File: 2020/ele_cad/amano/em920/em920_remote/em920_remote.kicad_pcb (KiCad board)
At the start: 2 copper layers, 40.6 x 58.4 mm, 8 parts, among them SW1 SW_Push, U1 ATtiny85-20PU, U2 TY92SS

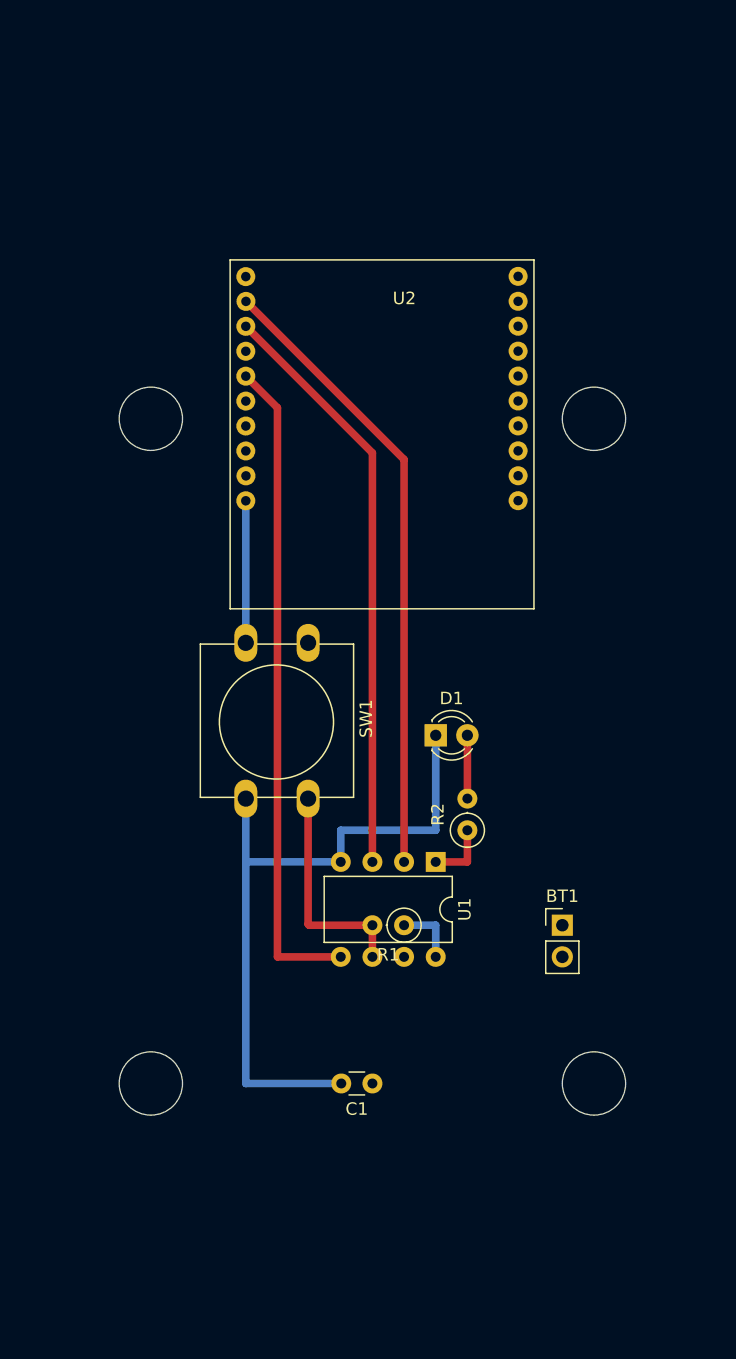
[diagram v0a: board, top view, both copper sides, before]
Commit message: 緊急停止リモコンのデータ更新
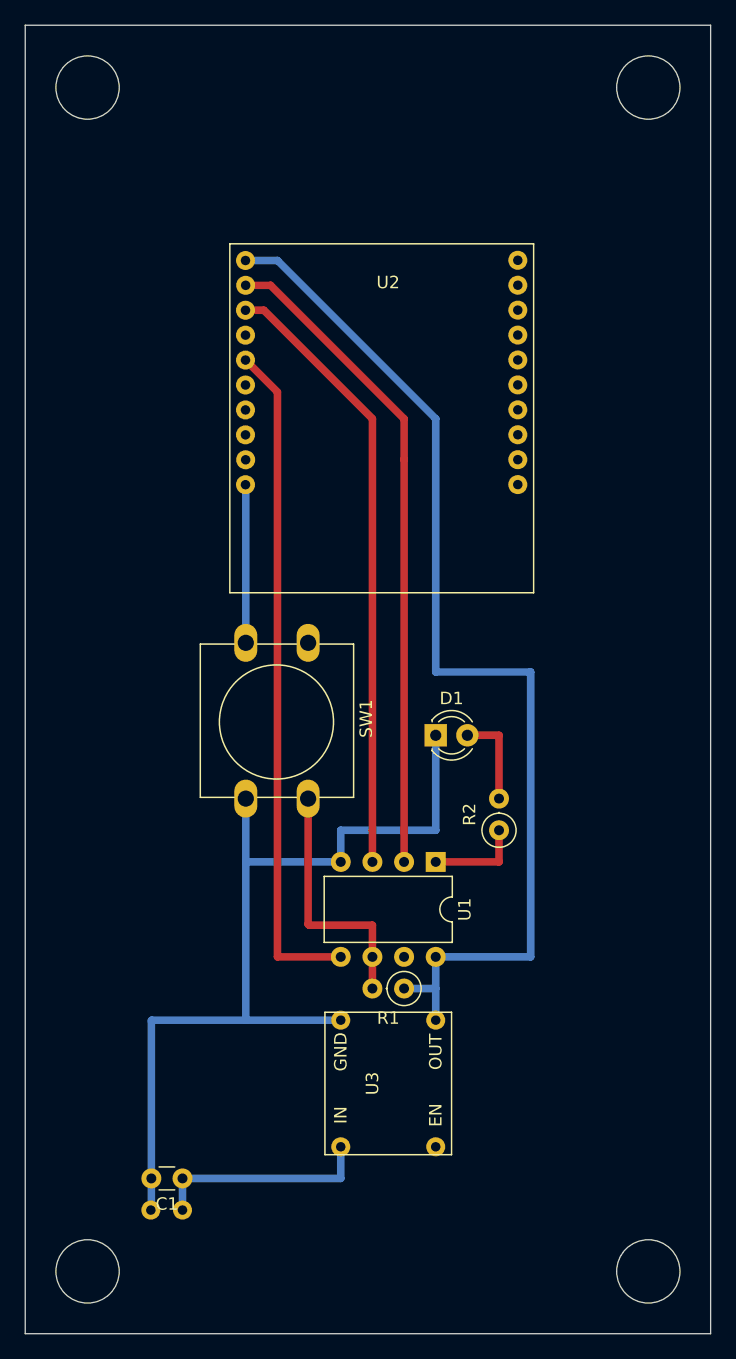
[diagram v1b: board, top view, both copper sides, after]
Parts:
- added U3: DCDC_3.3V, em920:DCDC_3.3V, F.Cu at (82.5, 153.0)
- BT1: footprint Connector_PinHeader_2.54mm:PinHeader_1x02_P2.54mm_Vertical -> em920:Battery_UM-4_2; moved to B.Cu
- moved BT1 23.4 mm to (96.5, 157.5), turned to 90 degrees
- moved C1 17.0 mm to (61.0, 154.9)
- moved R1 5.08 mm to (78.7, 139.7)
- moved R2 2.54 mm to (86.4, 127.0)
- moved U2 1.29 mm to (64.8, 107.9)
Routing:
- net +3V3: track 5.08 -> 86.6 mm
- net GND: track 67.3 -> 86.4 mm
- net +BATT: track 0.00 -> 17.8 mm
- net Net-(D1-Pad2): track 5.08 -> 7.62 mm
- net /LED1: track 5.08 -> 7.62 mm
- net /BTN1: track 17.8 -> 20.4 mm
- net /RX: track 50.2 -> 52.7 mm
- net /TX: track 47.2 -> 49.4 mm
- net /RESET: track 52.7 -> 54.0 mm
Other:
- board size 40.6 x 58.4 mm -> 55 x 105 mm
